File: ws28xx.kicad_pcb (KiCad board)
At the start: 4 copper layers, 28.6 x 63.5 mm, 48 parts, among them J1 Conn_02x03_Odd_Even, J2 Conn_02x03_Odd_Even, P1 USB_C_Plug, Q1 IRF8736, Q2 S8050, Q3 S8050, SW1 en, SW2 io0, U0 ESP32-PICO-D4, U1 LM1117-3.3, U2 74AXP2T3407, U4 STUSB4500QTR, U5 FT230XQ

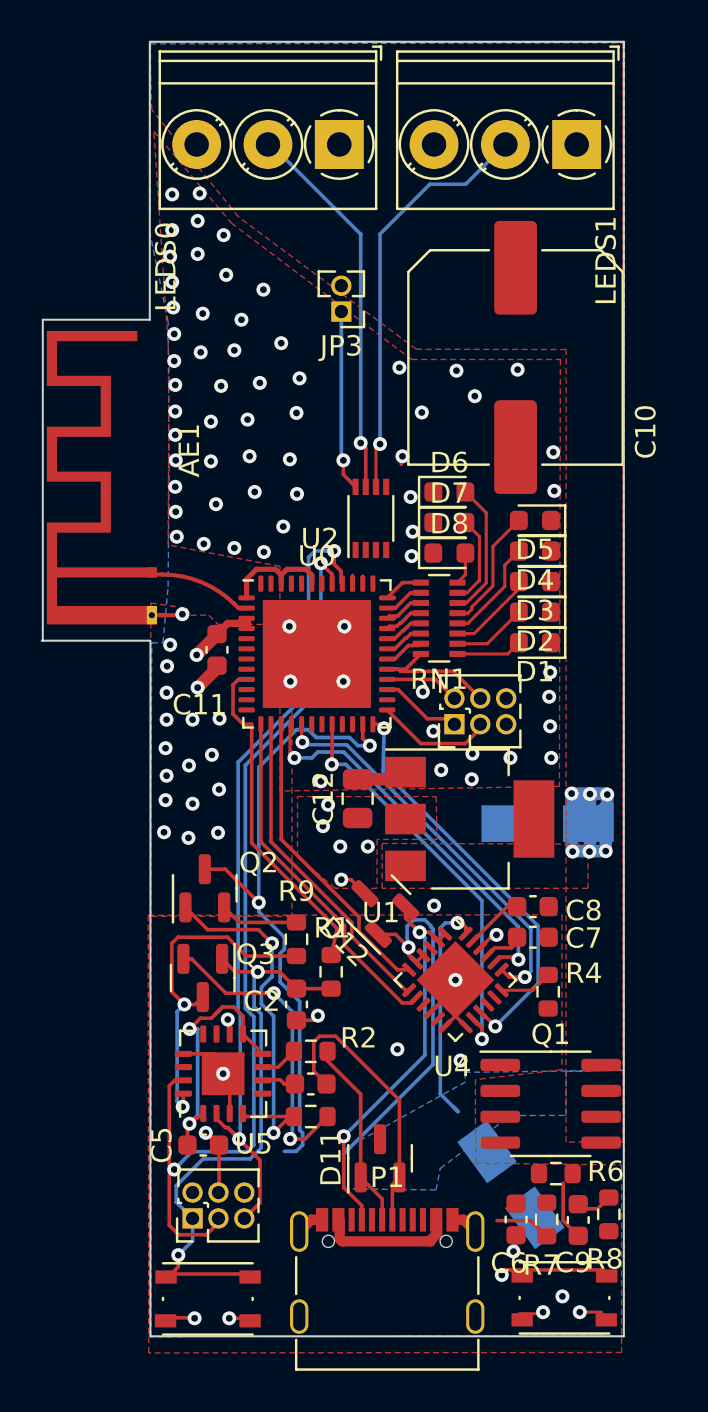
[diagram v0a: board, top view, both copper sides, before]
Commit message: routed
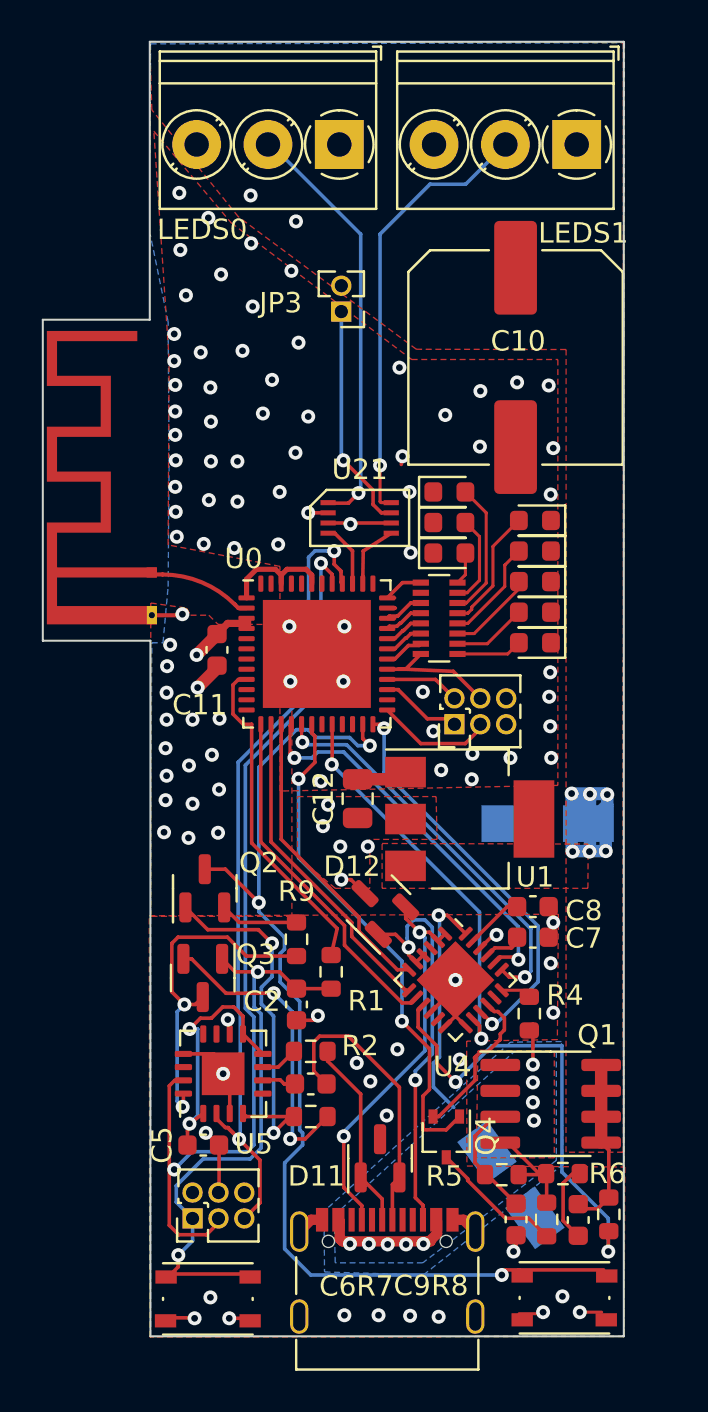
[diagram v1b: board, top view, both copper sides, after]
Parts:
- removed U2: 74AXP2T3407, precise:VSSOP-8_2.25x1.75mm_P0.5mm
- added Q4: DTC143E, Package_TO_SOT_SMD:SOT-323_SC-70, F.Cu at (127.5, 116.4)
- added R5: 100k, Resistor_SMD:R_0603_1608Metric, F.Cu at (130.2, 118.2)
- added U21: TXB0102, precise:SOIC-8, F.Cu at (123.2, 86.0)
- moved R4 1.42 mm to (131.5, 110.3)
- moved R6 0.35 mm to (133.2, 118.2)
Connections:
- U0 pad 18: unconnected-(U0-Pad18) -> power_en
- U4 pad 16: Net-(R7-Pad1) -> Net-(U4-Pad16)
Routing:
- net power_en: track 0.00 -> 25.3 mm, vias 0 -> 2
- net Net-(R8-Pad2): track 0.00 -> 22.6 mm, vias 0 -> 2
- net ESP_IO0: track 36.8 -> 52.5 mm
- net Net-(U4-Pad16): track 0.00 -> 7.87 mm
- net VDC: track 18.0 -> 25.8 mm, vias 1 -> 10
- net VBUS: track 17.9 -> 23.9 mm
- net Net-(Q1-Pad4): track 0.00 -> 5.03 mm
- net Net-(R7-Pad1): track 2.75 -> 6.58 mm
- net /LED_STRIP2: track 0.37 -> 3.60 mm
- net +3V3: track 5.60 -> 8.74 mm, vias 7 -> 8
- net /LED_STRIP1: track 0.40 -> 3.16 mm
- net Net-(JP3-Pad1): track 8.93 -> 11.2 mm
- net Net-(D12-Pad1): track 18.9 -> 20.8 mm, vias 1 -> 2
- net Net-(LEDS0-Pad2): track 18.7 -> 20.6 mm
- net /stat_led6: track 2.33 -> 0.77 mm
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- added copper zone on B.Cu, net VDC
- added copper zone on F.Cu, net VDC
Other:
- board size 28.6 x 63.5 mm -> 28.5 x 63.5 mm
